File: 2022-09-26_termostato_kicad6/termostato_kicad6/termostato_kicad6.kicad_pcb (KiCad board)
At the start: 2 copper layers, 13 parts, among them K1 SRD-05VDC-SL-C, Q1 BC337, U1 MCP6002-xP, X1 Power 5V, X2 OUT

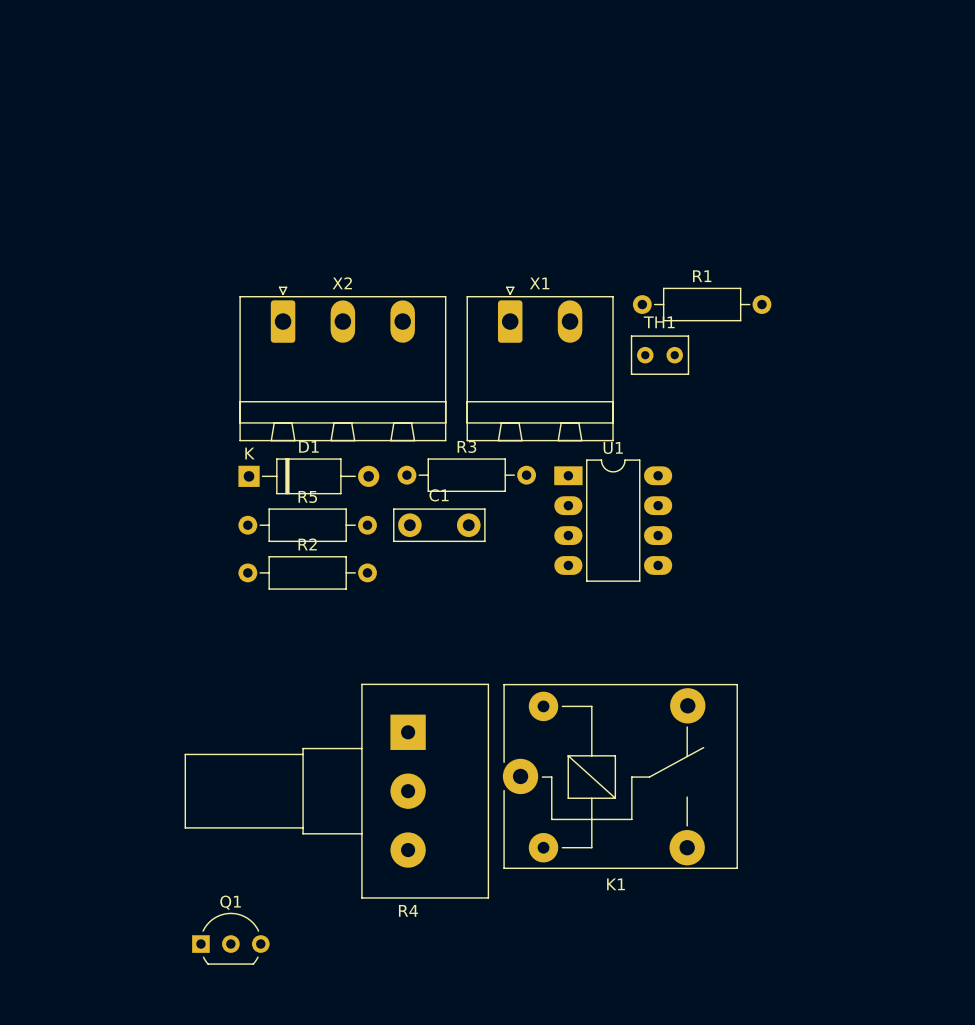
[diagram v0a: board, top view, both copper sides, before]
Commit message: layout
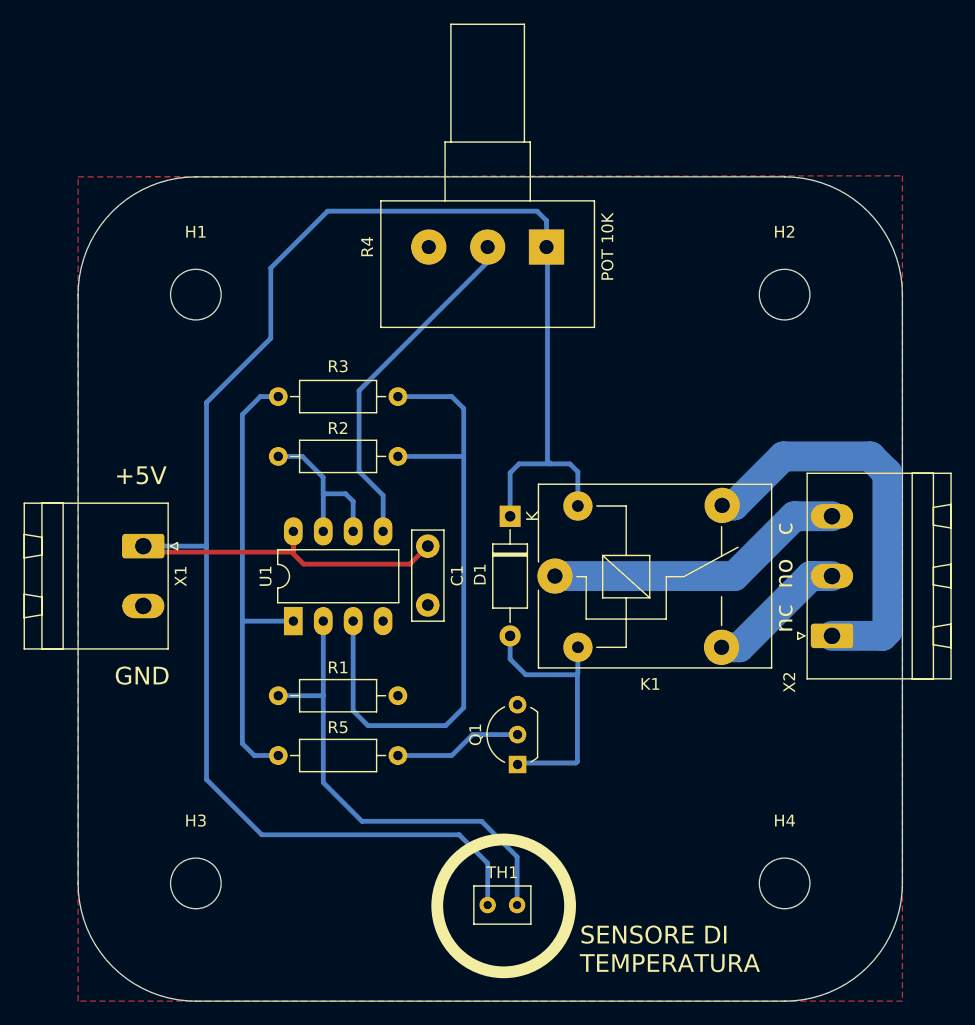
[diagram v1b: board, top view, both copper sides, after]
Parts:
- added H1: MountingHole, MountingHole:MountingHole_4.3mm_M4, F.Cu at (120.0, 65.0)
- added H2: MountingHole, MountingHole:MountingHole_4.3mm_M4, F.Cu at (170.0, 65.0)
- added H3: MountingHole, MountingHole:MountingHole_4.3mm_M4, F.Cu at (120.0, 115.0)
- added H4: MountingHole, MountingHole:MountingHole_4.3mm_M4, F.Cu at (170.0, 115.0)
- moved X2 53.7 mm to (174.0, 94.0), turned to 90 degrees
- moved TH1 48.6 mm to (144.8, 116.8)
- moved R1 45.4 mm to (127.0, 99.1)
- moved R4 42.9 mm to (149.8, 61.0), turned to -90 degrees
- moved X1 36.5 mm to (115.5, 86.4), turned to -90 degrees
- moved Q1 30.9 mm to (147.3, 104.9), turned to 90 degrees
- moved U1 26.4 mm to (128.3, 92.7), turned to 90 degrees
- moved D1 22.4 mm to (146.7, 83.8), turned to -90 degrees
- moved R5 19.7 mm to (127.0, 104.1)
- moved K1 17.3 mm to (150.5, 88.9)
- moved R2 10.2 mm to (127.0, 78.7)
- moved R3 6.72 mm to (137.2, 73.7), turned to 180 degrees
- moved C1 2.34 mm to (139.7, 86.4), turned to -90 degrees
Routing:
- net +5V: track 0.00 -> 170.1 mm
- net Net-(R2-Pad2): track 0.00 -> 55.2 mm
- net Net-(R1-Pad1): track 0.00 -> 40.7 mm
- net Vout: track 0.00 -> 39.4 mm
- net Net-(K1-Pad4): track 0.00 -> 34.6 mm
- net Net-(R4-Pad2): track 0.00 -> 29.5 mm
- net Net-(K1-Pad1): track 0.00 -> 25.6 mm
- net Net-(D1-Pad2): track 0.00 -> 23.1 mm
- net Vref: track 0.00 -> 14.5 mm
- net Net-(K1-Pad3): track 0.00 -> 11.9 mm
- net Net-(Q1-Pad2): track 0.00 -> 10.9 mm
- added copper zone on F.Cu, net GND
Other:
- board outline added: 70 x 70 mm
- board text added: "+5V"
- board text added: "GND"
- board text added: "SENSORE DI TEMPERATURA"
- board text added: "nc no c"
